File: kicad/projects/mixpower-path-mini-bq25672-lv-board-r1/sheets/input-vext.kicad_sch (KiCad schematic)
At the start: 7 parts, among them J4 VEXT, Q8 NTLJS17D0P03P8Z

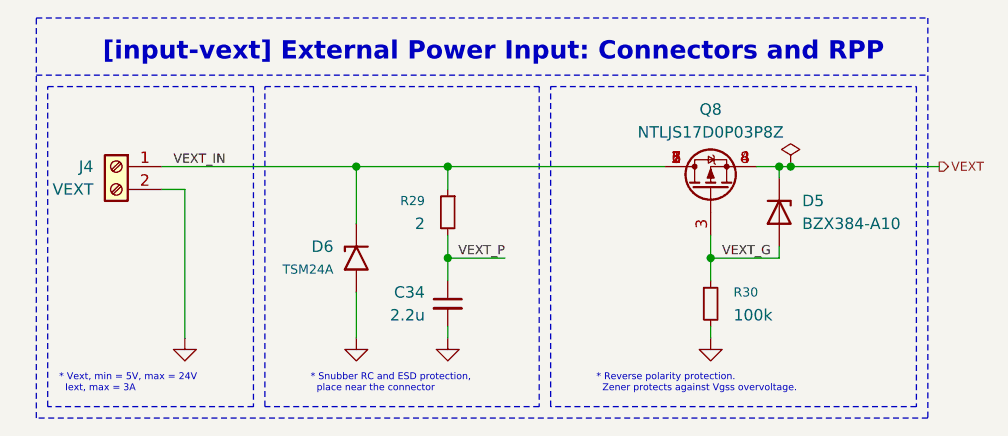
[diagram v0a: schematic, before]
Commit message: feat: small changes in schematics, some PCB routing
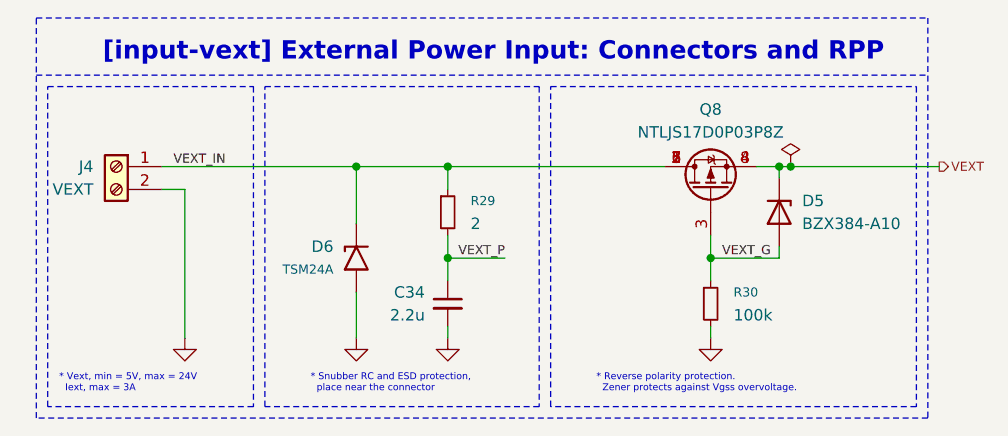
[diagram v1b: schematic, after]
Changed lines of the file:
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@@
 		(lib_id "Device:R_Small")
 		(at 113.03 63.5 0)
-		(mirror y)
 		(unit 1)
 		(exclude_from_sim no)
@@
 		(dnp no)
 		(property "Reference" "R29"
-			(at 110.49 62.2299 0)
+			(at 115.57 62.2299 0)
 			(effects
 				(font
@@
 		)
 		(property "Value" "2"
-			(at 110.49 64.7699 0)
+			(at 115.57 64.7699 0)
 			(effects
 				(font
@@
 		)
 		(instances
-			(project ""
+			(project "mixpower-path-mini-bq25672-lv-board-r1"
 				(path "/2e43857b-9bf9-460c-948c-ec2cf8a8d6b4/050b3b40-3e43-4f8a-9f9d-8e85b6cb1fd2"
 					(reference "J4")
@@
 		)
 		(instances
-			(project ""
+			(project "mixpower-path-mini-bq25672-lv-board-r1"
 				(path "/2e43857b-9bf9-460c-948c-ec2cf8a8d6b4/050b3b40-3e43-4f8a-9f9d-8e85b6cb1fd2"
 					(reference "D5")
@@
 		)
 		(instances
-			(project ""
+			(project "mixpower-path-mini-bq25672-lv-board-r1"
 				(path "/2e43857b-9bf9-460c-948c-ec2cf8a8d6b4/050b3b40-3e43-4f8a-9f9d-8e85b6cb1fd2"
 					(reference "D6")
@@
 		)
 		(instances
-			(project ""
+			(project "mixpower-path-mini-bq25672-lv-board-r1"
 				(path "/2e43857b-9bf9-460c-948c-ec2cf8a8d6b4/050b3b40-3e43-4f8a-9f9d-8e85b6cb1fd2"
 					(reference "Q8")

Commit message: feat: failed PCB routing
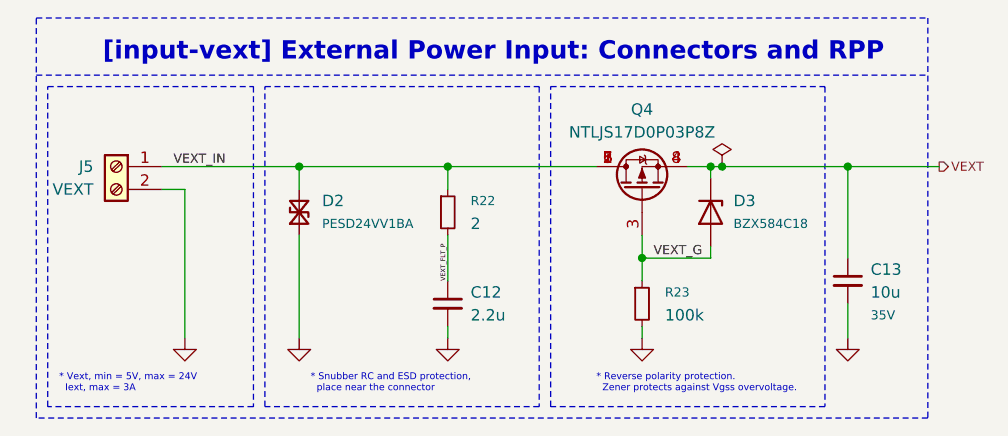
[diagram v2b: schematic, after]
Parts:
- removed D5: BZX384-A10, Diode_SMD:D_SOD-323, symbol Diode:BZX384xxxx
- removed D6: TSM24A, Package_TO_SOT_SMD:SOT-23, symbol Diode:TSM24A
- added C13: 10u, Capacitor_SMD:C_0402_1005Metric, symbol Device:C_Small
- added D2: PESD24VV1BA, Diode_SMD:D_SOD-323, symbol Device:D_TVS_Small
- added D3: BZX584C18, Diode_SMD:D_SOD-523, symbol Diode:DZ2S180X0L
- C12: renamed from C34; footprint Capacitor_SMD:C_0603_1608Metric -> Resistor_SMD:R_0402_1005Metric
- renumbered J4 to J5, Q8 to Q4, R29 to R22, R30 to R23
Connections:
- net GND: now also C13.2, D2.1 (A1)
- net VEXT: now also C13.1, D3.1 (K)
- net VEXT_G: now also D3.2 (A)
- net VEXT_IN: now also D2.2 (A2)
- net VEXT_P renamed VEXT_FLT_P
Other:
- moved on the sheet: Q4, R23
